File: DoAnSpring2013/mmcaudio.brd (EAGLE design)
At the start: 181.9 x 121.9 mm, 84 parts, among them IC1 TL082, IC2 TL082, IC3 LM1117, IC4 TL082, IC5 TL082, U1 DAC0808LCN, U2 TEA2025B, X1 HD44780LCD-1602

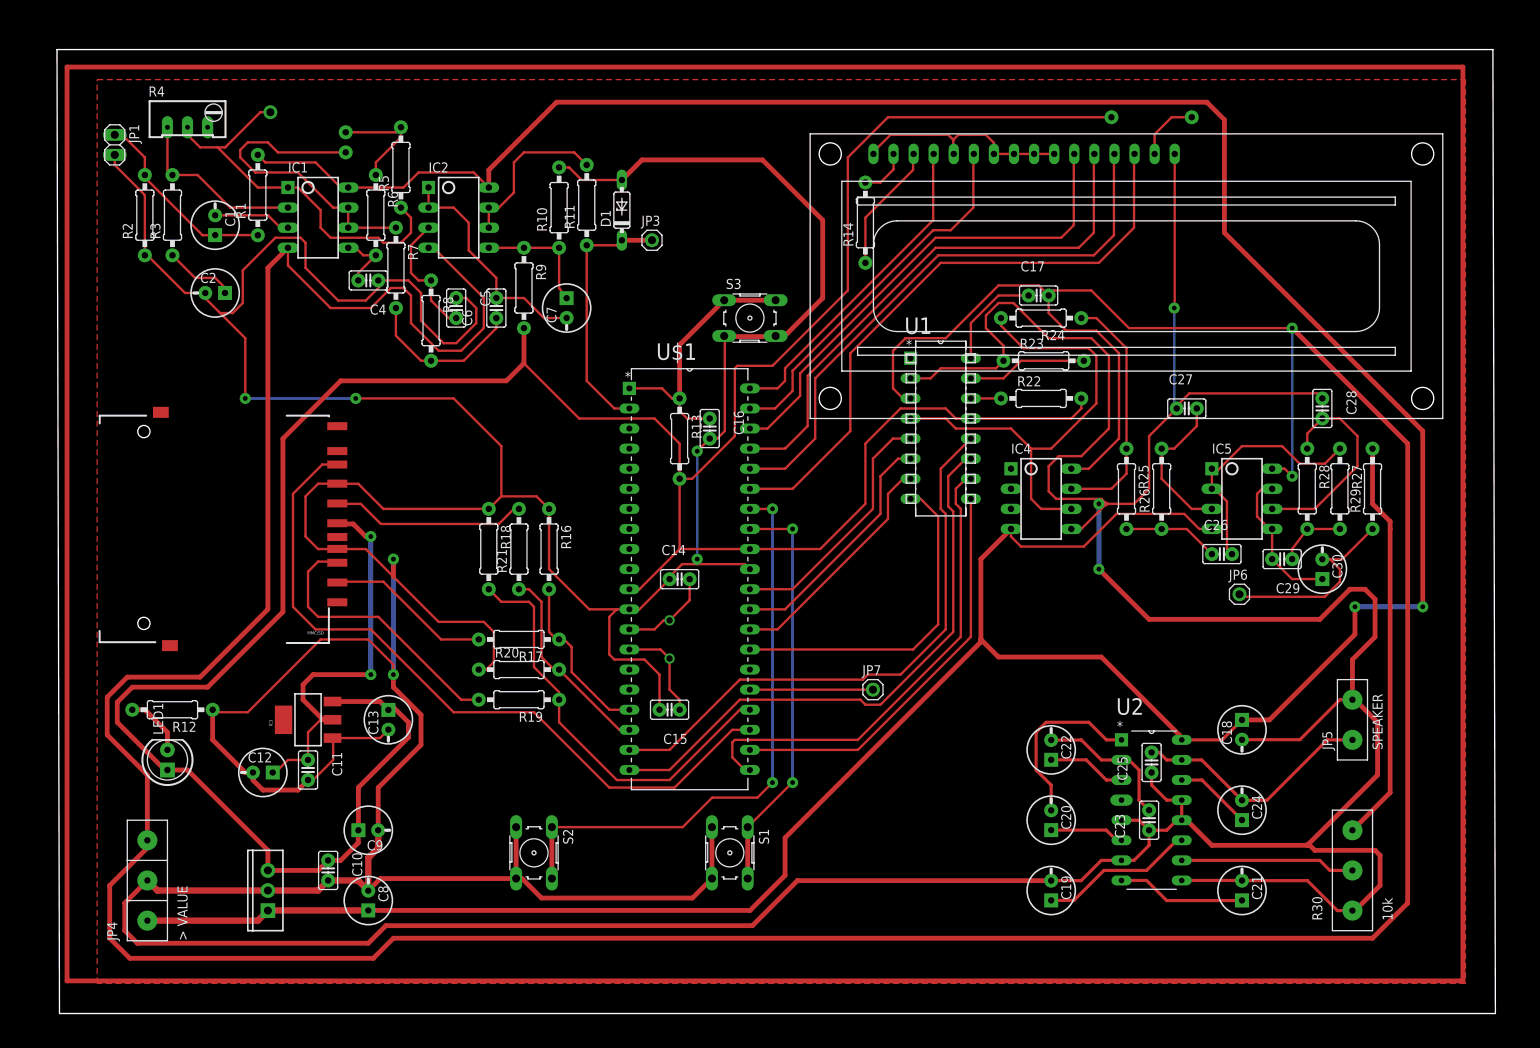
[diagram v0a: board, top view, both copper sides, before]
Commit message: clean the fault
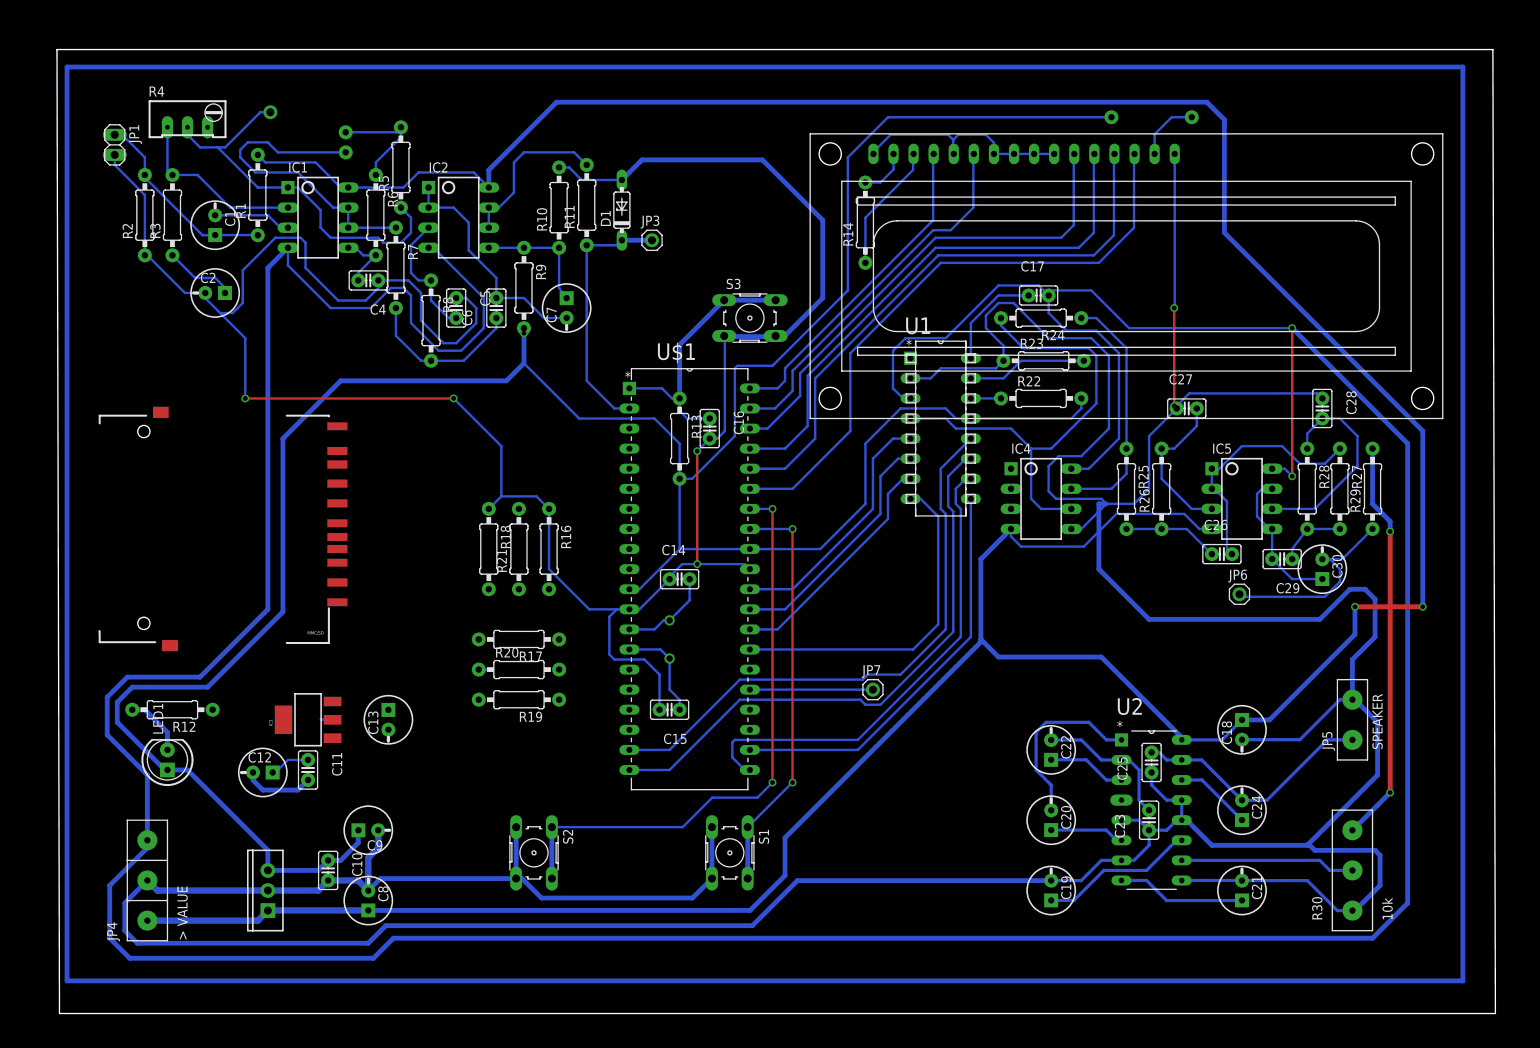
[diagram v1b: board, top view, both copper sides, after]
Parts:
- R16, R18, R20: value 6.8k -> 3.3k
- R17, R19, R21: value 6.8k -> 2.2k
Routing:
- net GND: track 1028.6 -> 869.7 mm, vias 9 -> 6
- net MISO: track 91.7 -> 0.00 mm
- net MOSI: track 53.4 -> 0.00 mm
- net +3V3: track 50.6 -> 6.63 mm, vias 2 -> 0
- net N$38: track 35.2 -> 0.00 mm
- net VCC: track 362.5 -> 330.8 mm, vias 0 -> 1
- net CLK: track 25.4 -> 0.00 mm
- net N$40: track 24.8 -> 0.00 mm
- net CS: track 21.5 -> 0.00 mm
- net N$36: track 21.0 -> 0.00 mm
- net N$30: track 56.0 -> 51.2 mm, vias 0 -> 2
- removed copper zone on layer 1, net GND

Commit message: done 2311
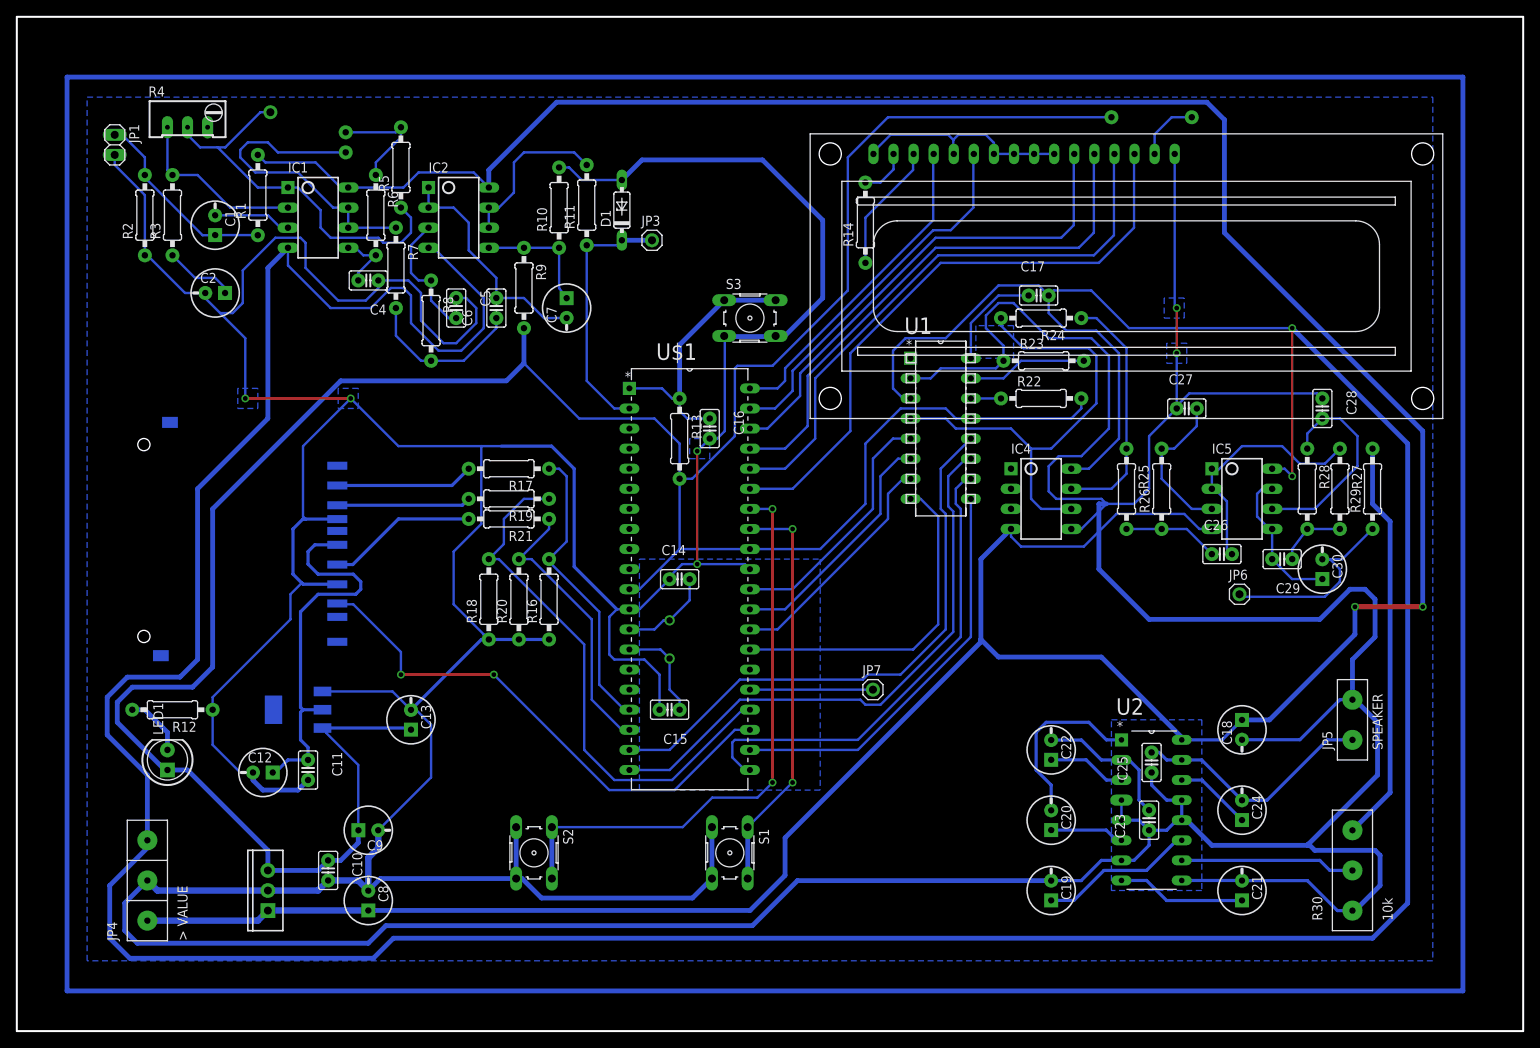
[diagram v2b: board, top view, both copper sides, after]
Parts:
- moved R19 25.4 mm to (71.1, 86.4)
- moved R17 21.6 mm to (71.1, 90.2)
- moved R20 8.89 mm to (72.4, 73.7), turned to 90 degrees
- moved R16 6.35 mm to (76.2, 73.7), turned to 90 degrees
- moved R18 6.35 mm to (68.6, 73.7), turned to 90 degrees
- moved R21 4.02 mm to (71.1, 83.8), turned to 180 degrees
- moved C13 2.86 mm to (58.7, 58.4), turned to 270 degrees
- moved IC3 1.80 mm to (44.5, 59.7), flipped to the bottom, turned to 270 degrees
- moved MMC/SD 1.27 mm to (48.3, 81.3), flipped to the bottom, turned to 0 degrees
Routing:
- net GND: track 869.7 -> 1015.9 mm
- net MOSI: track 0.00 -> 68.7 mm
- net MISO: track 0.00 -> 66.8 mm, vias 0 -> 2
- net +3V3: track 6.63 -> 50.0 mm
- net CS: track 0.00 -> 37.6 mm
- net CLK: track 0.00 -> 35.5 mm
- net VCC: track 330.8 -> 355.6 mm, vias 1 -> 0
- net N$40: track 0.00 -> 19.0 mm
- net N$36: track 0.00 -> 17.5 mm
- net N$38: track 0.00 -> 17.0 mm
- net -12V: track 520.8 -> 519.3 mm
- net N$30: vias 2 -> 0
- added copper zone on layer 16, net GND
- added copper zone on layer 16, net N$20
- added copper zone on layer 16, net N$35
- added copper zone on layer 16, net N$39
- added copper zone on layer 16, net N$41
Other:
- board size 181.9 x 121.9 mm -> 190.5 x 128.3 mm
